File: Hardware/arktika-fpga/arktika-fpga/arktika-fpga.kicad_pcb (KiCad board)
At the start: 4 copper layers, 131.8 x 90.1 mm, 129 parts

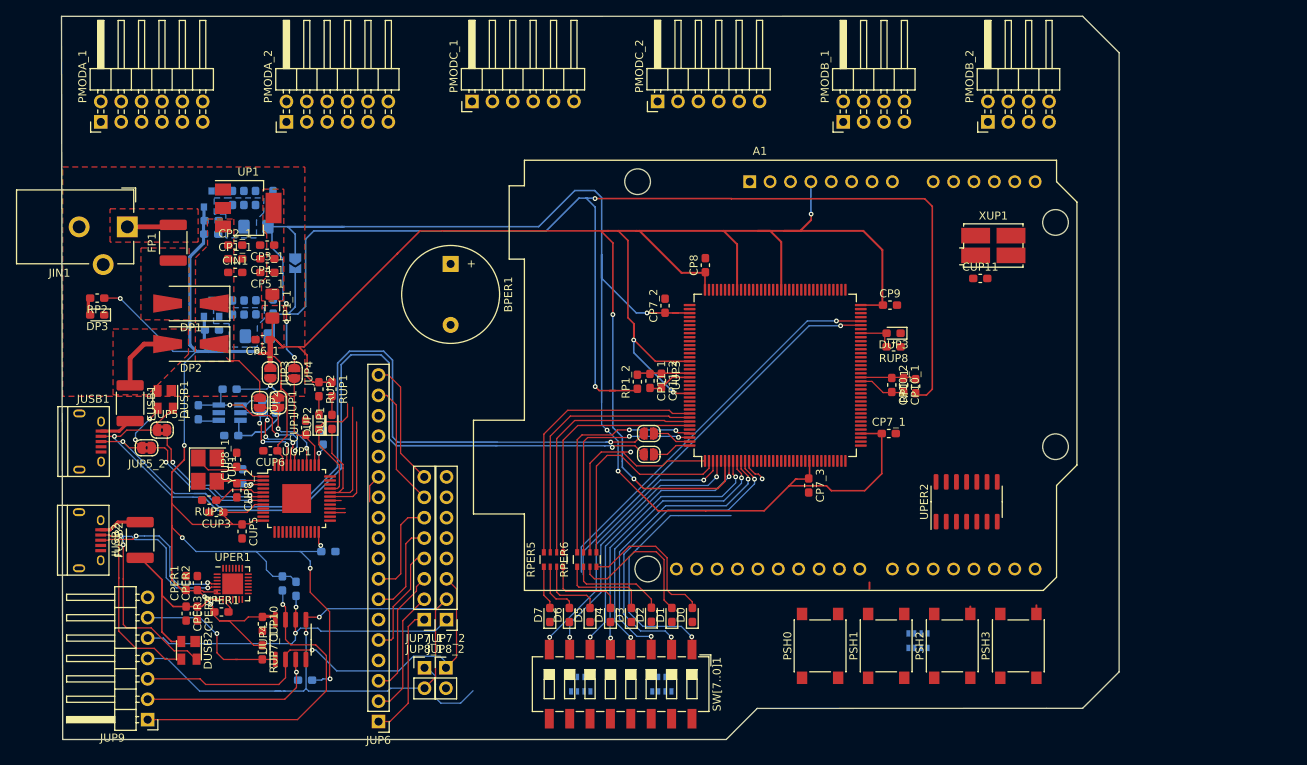
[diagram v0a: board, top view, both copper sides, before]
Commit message: Major routing updates. Did work on silkscreen. Optimized io placing. Misc changes
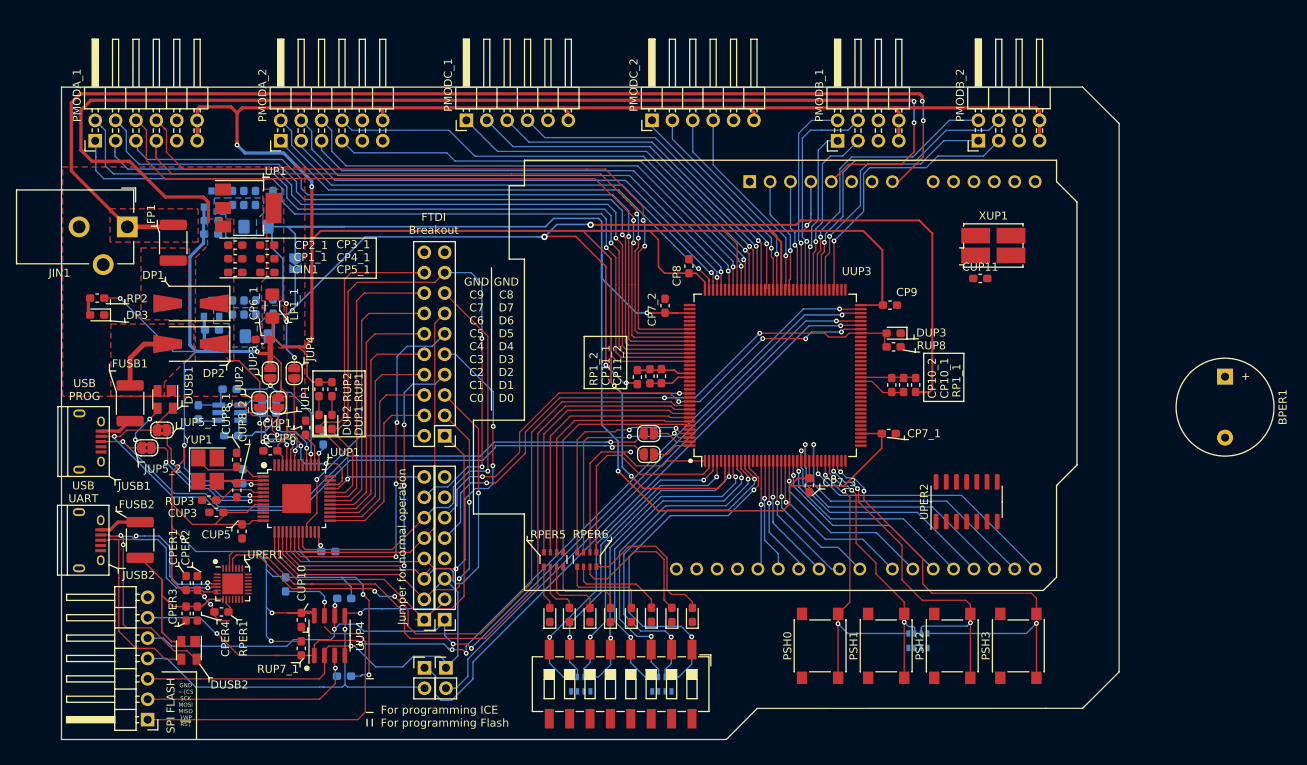
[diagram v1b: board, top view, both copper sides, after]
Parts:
- A1: footprint Module:Arduino_UNO_R3_WithMountingHoles -> Module:Arduino_UNO_R3
- JUP6: value Conn_01x18 -> Conn_02x10_Odd_Even; footprint Pin_Headers:Pin_Header_Straight_1x18_Pitch2.54mm -> Connector_PinHeader_2.54mm:PinHeader_2x10_P2.54mm_Vertical
- PMODA_1, PMODA_2: value Conn_02x06_Top_Bottom -> Conn_02x06_Odd_Even
- moved BPER1 97.5 mm to (229.3, 93.7)
- moved JUP6 36.5 mm to (132.1, 101.0)
- moved RUP7_4 6.12 mm to (119.5, 121.3), turned to 180 degrees
- moved RUP7_2 4.88 mm to (119.5, 131.0)
- moved RUP7_1 4.88 mm to (114.2, 127.5)
- moved CUP10 4.88 mm to (114.2, 124.0)
- moved UUP4 4.88 mm to (117.7, 125.9)
- moved PMODB_2 2.62 mm to (198.6, 64.3)
- moved PMODA_1 2.45 mm to (88.5, 64.3)
- moved PMODA_2 2.45 mm to (111.7, 64.3)
- moved PMODB_1 2.45 mm to (181.0, 64.3)
- moved PMODC_1 2.45 mm to (134.8, 61.7)
- moved PMODC_2 2.45 mm to (157.9, 61.7)
- moved CP8 2.05 mm to (162.5, 79.9)
- moved CP11_1 0.58 mm to (157.6, 93.6)
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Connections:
- net Net-(JUP6-Pad1) renamed /USB AND PROG/ADBUS0
- net Net-(JUP6-Pad16) renamed /USB AND PROG/ACBUS7
- CP7_3 pad 1: Net-(CP7_3-Pad1) -> /Power/VCC_CORE
- CUP11 pad 1: /FPGA_IO/3V3 -> /VCC3V3
- JUP6 pad 10: Net-(JUP6-Pad10) -> /USB AND PROG/ACBUS4
- JUP6 pad 11: Net-(JUP6-Pad11) -> /USB AND PROG/ADBUS5
- JUP6 pad 12: Net-(JUP6-Pad12) -> /USB AND PROG/ACBUS5
- JUP6 pad 13: Net-(JUP6-Pad13) -> /USB AND PROG/ADBUS6
- JUP6 pad 14: Net-(JUP6-Pad14) -> /USB AND PROG/ACBUS6
- JUP6 pad 15: Net-(JUP6-Pad15) -> /USB AND PROG/ADBUS7
- JUP6 pad 2: Net-(JUP6-Pad2) -> /USB AND PROG/ACBUS0
- JUP6 pad 3: Net-(JUP6-Pad3) -> /USB AND PROG/ADBUS1
- JUP6 pad 4: Net-(JUP6-Pad4) -> /USB AND PROG/ACBUS1
- JUP6 pad 5: Net-(JUP6-Pad5) -> /USB AND PROG/ADBUS2
- JUP6 pad 6: Net-(JUP6-Pad6) -> /USB AND PROG/ACBUS2
- JUP6 pad 7: Net-(JUP6-Pad7) -> /USB AND PROG/ADBUS3
- JUP6 pad 8: Net-(JUP6-Pad8) -> /USB AND PROG/ACBUS3
- JUP6 pad 9: Net-(JUP6-Pad9) -> /USB AND PROG/ADBUS4
- JUP7_1 pad 2: Net-(JUP6-Pad2) -> /USB AND PROG/ADBUS1
- JUP7_1 pad 3: Net-(JUP6-Pad3) -> /USB AND PROG/ADBUS2
- JUP7_1 pad 4: Net-(JUP6-Pad5) -> /USB AND PROG/ADBUS4
- JUP7_1 pad 5: Net-(JUP6-Pad7) -> /USB AND PROG/ADBUS6
- JUP7_1 pad 6: Net-(JUP6-Pad8) -> /USB AND PROG/ADBUS7
- PMODA_1 pad 10: /FPGA_IO/PMOD1_A_10 -> GND
- PMODA_1 pad 11: GND -> /VCC3V3
- PMODA_1 pad 12: /FPGA_IO/3V3 -> /VCC3V3
- PMODA_1 pad 2: /FPGA_IO/PMOD1_A_2 -> /FPGA_IO/PMOD1_A_7
- PMODA_1 pad 3: /FPGA_IO/PMOD1_A_3 -> /FPGA_IO/PMOD1_A_2
- PMODA_1 pad 4: /FPGA_IO/PMOD1_A_4 -> /FPGA_IO/PMOD1_A_8
- PMODA_1 pad 5: GND -> /FPGA_IO/PMOD1_A_3
- PMODA_1 pad 6: /FPGA_IO/3V3 -> /FPGA_IO/PMOD1_A_9
- PMODA_1 pad 7: /FPGA_IO/PMOD1_A_7 -> /FPGA_IO/PMOD1_A_4
- PMODA_1 pad 8: /FPGA_IO/PMOD1_A_8 -> /FPGA_IO/PMOD1_A_10
- PMODA_1 pad 9: /FPGA_IO/PMOD1_A_9 -> GND
- PMODA_2 pad 10: /FPGA_IO/PMOD1_B_10 -> GND
- PMODA_2 pad 11: GND -> /VCC3V3
- PMODA_2 pad 12: /FPGA_IO/3V3 -> /VCC3V3
- PMODA_2 pad 2: /FPGA_IO/PMOD1_B_2 -> /FPGA_IO/PMOD1_B_7
- PMODA_2 pad 3: /FPGA_IO/PMOD1_B_3 -> /FPGA_IO/PMOD1_B_2
- PMODA_2 pad 4: /FPGA_IO/PMOD1_B_4 -> /FPGA_IO/PMOD1_B_8
- PMODA_2 pad 5: GND -> /FPGA_IO/PMOD1_B_3
- PMODA_2 pad 6: /FPGA_IO/3V3 -> /FPGA_IO/PMOD1_B_9
- PMODA_2 pad 7: /FPGA_IO/PMOD1_B_7 -> /FPGA_IO/PMOD1_B_4
- PMODA_2 pad 8: /FPGA_IO/PMOD1_B_8 -> /FPGA_IO/PMOD1_B_10
- PMODA_2 pad 9: /FPGA_IO/PMOD1_B_9 -> GND
- PMODB_1 pad 7: /FPGA_IO/3V3 -> /VCC3V3
- PMODB_1 pad 8: /FPGA_IO/3V3 -> /VCC3V3
- PMODB_2 pad 1: /FPGA_IO/PMOD2_A_1 -> /FPGA_IO/PMOD2_B_1
- PMODB_2 pad 7: /FPGA_IO/3V3 -> /VCC3V3
- PMODB_2 pad 8: /FPGA_IO/3V3 -> /VCC3V3
- PMODC_1 pad 6: /FPGA_IO/3V3 -> /VCC3V3
- PMODC_2 pad 6: /FPGA_IO/3V3 -> /VCC3V3
- UUP1 pad 14: Net-(JUP6-Pad2) -> /USB AND PROG/ADBUS1
- UUP1 pad 15: Net-(JUP6-Pad3) -> /USB AND PROG/ADBUS2
- UUP1 pad 16: Net-(JUP6-Pad4) -> /USB AND PROG/ADBUS3
- UUP1 pad 17: Net-(JUP6-Pad5) -> /USB AND PROG/ADBUS4
- UUP1 pad 18: Net-(JUP6-Pad6) -> /USB AND PROG/ADBUS5
- UUP1 pad 19: Net-(JUP6-Pad7) -> /USB AND PROG/ADBUS6
- UUP1 pad 20: Net-(JUP6-Pad8) -> /USB AND PROG/ADBUS7
- UUP1 pad 21: Net-(JUP6-Pad9) -> /USB AND PROG/ACBUS0
- UUP1 pad 25: Net-(JUP6-Pad10) -> /USB AND PROG/ACBUS1
- UUP1 pad 26: Net-(JUP6-Pad11) -> /USB AND PROG/ACBUS2
- UUP1 pad 27: Net-(JUP6-Pad12) -> /USB AND PROG/ACBUS3
- UUP1 pad 28: Net-(JUP6-Pad13) -> /USB AND PROG/ACBUS4
- UUP1 pad 29: Net-(JUP6-Pad14) -> /USB AND PROG/ACBUS5
- UUP1 pad 30: Net-(JUP6-Pad15) -> /USB AND PROG/ACBUS6
- UUP3 pad 102: /FPGA_IO/PMOD1_B_10 -> /FPGA_IO/PMOD1_B_3
- UUP3 pad 104: /FPGA_IO/PMOD1_B_1 -> /FPGA_IO/PMOD1_B_8
- UUP3 pad 106: /FPGA_IO/PMOD1_B_3 -> /FPGA_IO/PMOD1_B_7
- UUP3 pad 107: /FPGA_IO/PMOD1_B_4 -> /FPGA_IO/PMOD1_B_1
- UUP3 pad 115: /FPGA_IO/PMOD1_A_1 -> /FPGA_IO/PMOD1_A_10
- UUP3 pad 116: /FPGA_IO/PMOD1_A_2 -> /FPGA_IO/PMOD1_A_4
- UUP3 pad 117: /FPGA_IO/PMOD1_A_3 -> /FPGA_IO/PMOD1_A_9
- UUP3 pad 118: /FPGA_IO/PMOD1_A_4 -> /FPGA_IO/PMOD1_A_3
- UUP3 pad 119: /FPGA_IO/PMOD1_A_7 -> /FPGA_IO/PMOD1_A_8
- UUP3 pad 120: /FPGA_IO/PMOD1_A_8 -> /FPGA_IO/PMOD1_A_2
- UUP3 pad 121: /FPGA_IO/PMOD1_A_9 -> /FPGA_IO/PMOD1_A_7
- UUP3 pad 122: /FPGA_IO/PMOD1_A_10 -> /FPGA_IO/PMOD1_A_1
- UUP3 pad 73: /FPGA_IO/PMOD2_B_3 -> Net-(UUP3-Pad73)
- UUP3 pad 74: /FPGA_IO/PMOD2_A_1 -> Net-(UUP3-Pad74)
- UUP3 pad 75: /FPGA_IO/PMOD2_B_4 -> Net-(UUP3-Pad75)
- UUP3 pad 76: /FPGA_IO/PMOD2_B_2 -> /FPGA_IO/PMOD2_B_3
- UUP3 pad 78: /FPGA_IO/PMOD2_A_3 -> /FPGA_IO/PMOD2_B_1
- UUP3 pad 79: /FPGA_IO/PMOD2_A_1 -> /FPGA_IO/PMOD2_B_4
- UUP3 pad 80: /FPGA_IO/PMOD2_A_4 -> /FPGA_IO/PMOD2_B_2
- UUP3 pad 81: /FPGA_IO/PMOD2_A_2 -> /FPGA_IO/PMOD2_A_3
- UUP3 pad 82: Net-(UUP3-Pad82) -> /FPGA_IO/PMOD2_A_1
- UUP3 pad 83: Net-(UUP3-Pad83) -> /FPGA_IO/PMOD2_A_4
- UUP3 pad 84: Net-(UUP3-Pad84) -> /FPGA_IO/PMOD2_A_2
- UUP3 pad 85: Net-(UUP3-Pad85) -> /FPGA_IO/ARDUINO_RESET
- UUP3 pad 87: Net-(UUP3-Pad87) -> /FPGA_IO/ARDUINO_EXTRA_1
- UUP3 pad 88: /FPGA_IO/PMOD3_A_4 -> /FPGA_IO/PMOD3_B_4
- UUP3 pad 90: /FPGA_IO/PMOD3_A_3 -> /FPGA_IO/PMOD3_B_3
- UUP3 pad 91: /FPGA_IO/PMOD3_A_2 -> /FPGA_IO/PMOD3_B_2
- UUP3 pad 93: /FPGA_IO/PMOD3_A_1 -> /FPGA_IO/PMOD3_B_1
- UUP3 pad 94: /FPGA_IO/PMOD3_B_4 -> /FPGA_IO/PMOD3_A_4
- UUP3 pad 95: /FPGA_IO/PMOD3_B_3 -> /FPGA_IO/PMOD3_A_3
- UUP3 pad 96: /FPGA_IO/PMOD3_B_2 -> /FPGA_IO/PMOD3_A_2
- UUP3 pad 97: /FPGA_IO/PMOD3_B_1 -> /FPGA_IO/PMOD3_A_1
- UUP3 pad 98: /FPGA_IO/PMOD1_B_7 -> /FPGA_IO/PMOD1_B_10
- UUP3 pad 99: /FPGA_IO/PMOD1_B_8 -> /FPGA_IO/PMOD1_B_4
- XUP1 pad 4: /FPGA_IO/3V3 -> /VCC3V3
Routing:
- net /VCC3V3: track 426.3 -> 605.8 mm, vias 15 -> 20
- net /VCC5V: track 7.56 -> 156.1 mm, vias 0 -> 2
- net /VIN: track 5.79 -> 143.5 mm, vias 0 -> 2
- net /FPGA_IO/PMOD1_A_7: track 0.00 -> 98.6 mm, vias 0 -> 1
- net /FPGA_IO/PMOD1_A_1: track 0.00 -> 97.6 mm, vias 0 -> 1
- net /FPGA_IO/PMOD1_A_8: track 0.00 -> 94.9 mm, vias 0 -> 1
- net /FPGA_IO/PMOD1_A_2: track 0.00 -> 93.6 mm, vias 0 -> 1
- net /USB AND PROG/FLASH_CS: track 19.7 -> 112.3 mm, vias 1 -> 5
- net /FPGA_IO/PMOD1_A_9: track 0.00 -> 91.3 mm, vias 0 -> 2
- net /FPGA_IO/PMOD1_A_3: track 0.00 -> 90.0 mm, vias 0 -> 1
- net /FPGA_IO/PMOD1_A_10: track 0.00 -> 88.8 mm, vias 0 -> 2
- net UART_TX: track 0.00 -> 88.4 mm
- net /FPGA_IO/PMOD1_A_4: track 0.00 -> 87.2 mm, vias 0 -> 2
- net UART_RX: track 0.00 -> 86.8 mm, vias 0 -> 2
- net /USB AND PROG/ICE_SCK: track 44.0 -> 116.4 mm, vias 2 -> 5
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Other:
- board size 131.8 x 90.1 mm -> 131.8 x 81.3 mm
- board text added: "FTDI Breakout"
- board text added: "For programming ICE For programming Flash"
- board text added: "GND C8 D7 D6 D5 D4 D3 D2 D1 D0"
- board text added: "GND C9 C7 C6 C5 C4 C3 C2 C1 C0"
- board text added: "GND ~CS SCK MOSI MISO ~WP ~RST"
- board text added: "Jumper for normal operation"
- board text added: "SPI FLASH"
- board text added: "USB PROG"
- board text added: "USB UART"
